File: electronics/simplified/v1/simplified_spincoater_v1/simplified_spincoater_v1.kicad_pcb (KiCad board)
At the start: 6 copper layers, 49.7 x 49.6 mm, 91 parts, among them U1 HUSB238A-BB001-QN16R, U10 TJA1051TK/3, U11 NTTFS5C454NL, U13 NTTFS5C454NL, U14 NTTFS5C454NL, U15 NTTFS5C454NL, U16 NTTFS5C454NL, U17 NTTFS5C454NL, U18 TJA1051TK/3, U2 LMR51420YDD, U3 TPS62933DRL, U4 GT-USB-7004N, U6 ESP32-S3-WROOM-1, U7 STM32G474VEH6, U8 DRV8323SRTA, U9 AS5600

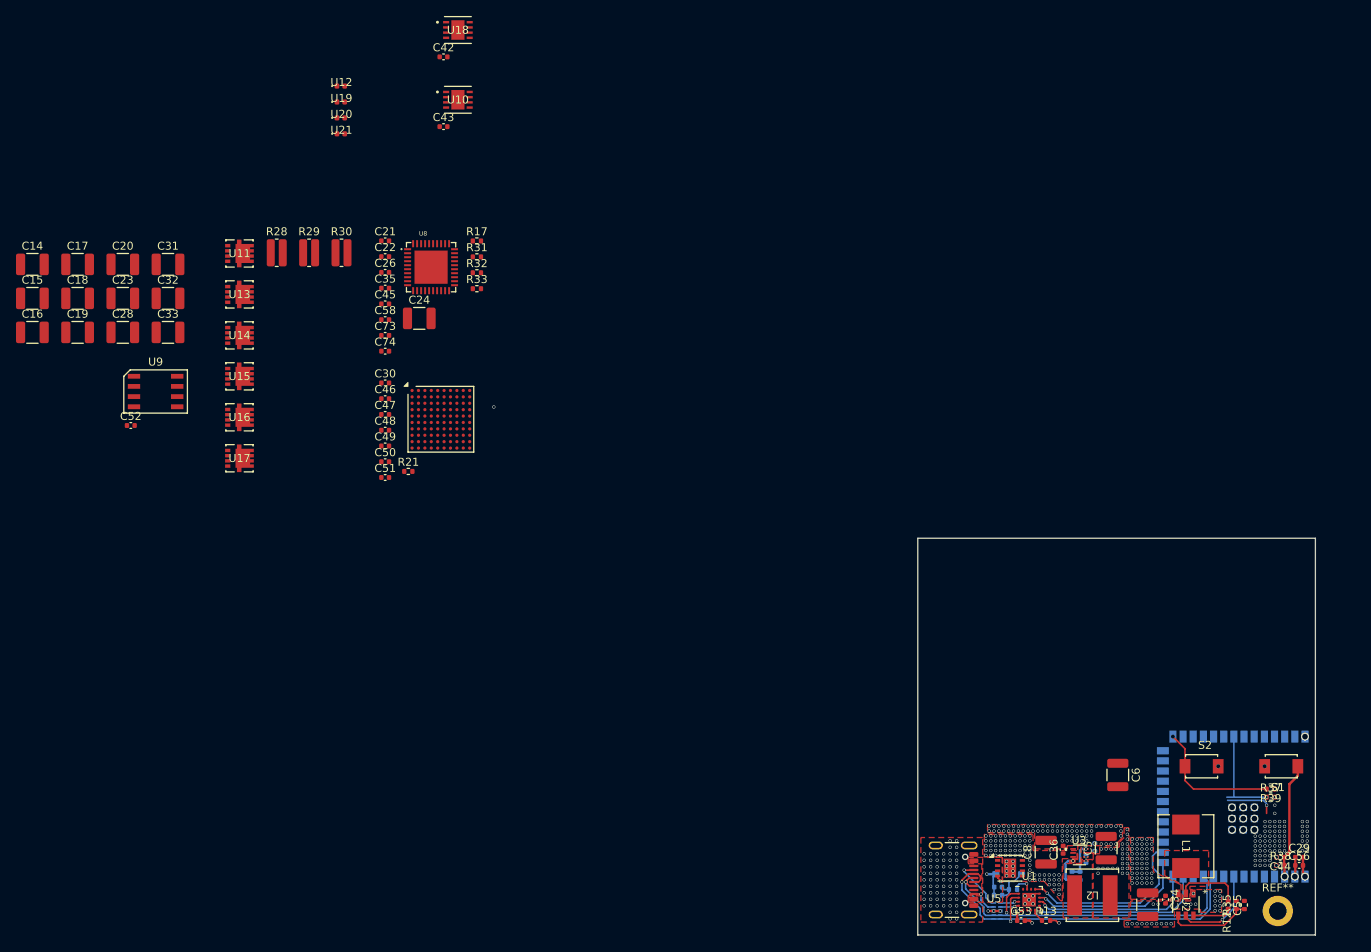
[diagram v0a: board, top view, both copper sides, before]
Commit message: fix
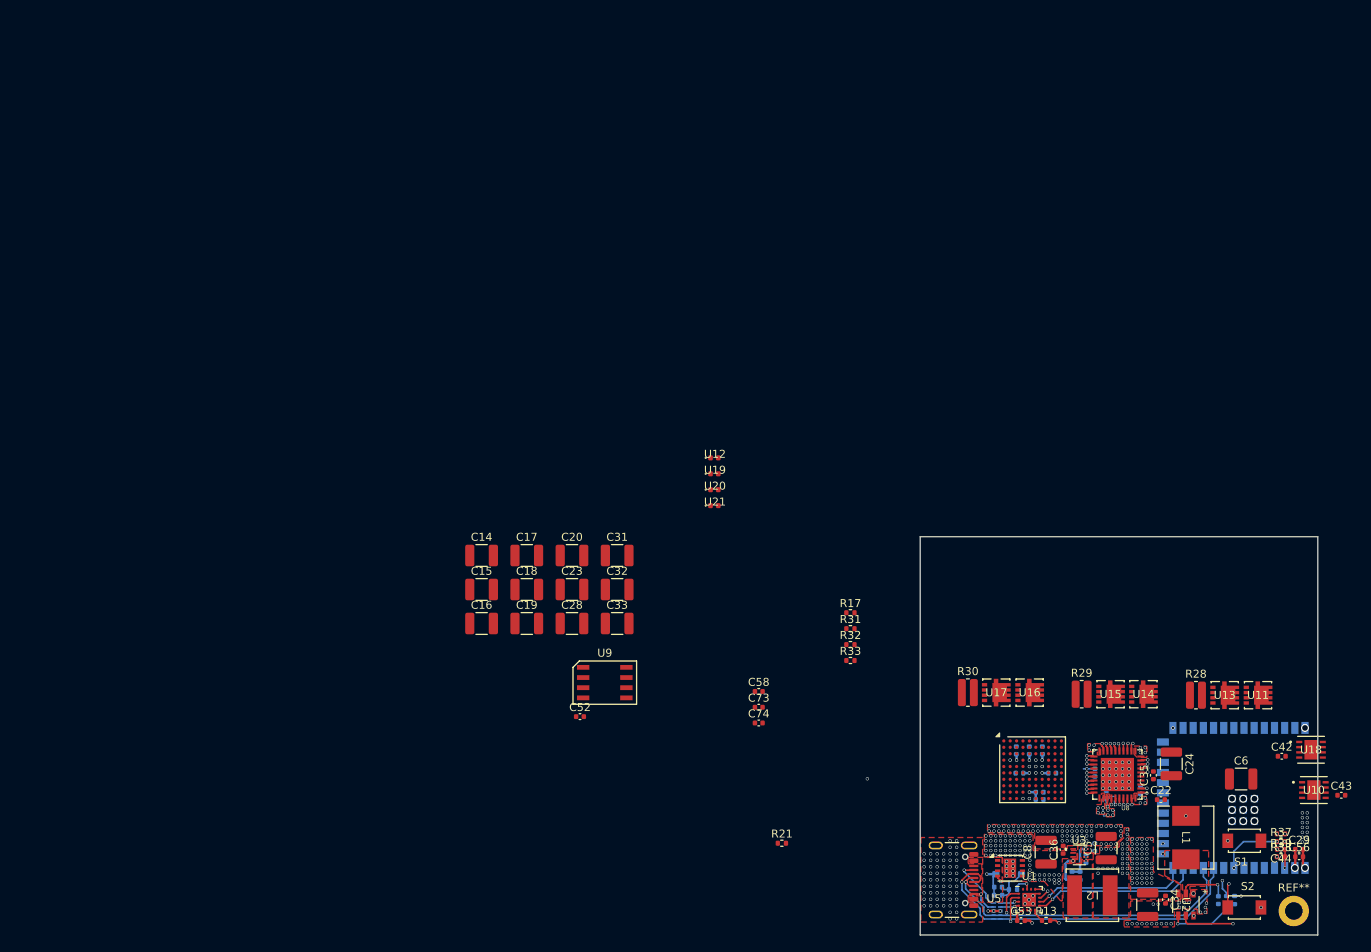
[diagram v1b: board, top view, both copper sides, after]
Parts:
- C21, C26, C30, C45, C46, C47, C48, C49, C50, C51, C55, R12, R35: moved to B.Cu
- moved C43 139.9 mm to (165.9, 97.5)
- moved U18 139.5 mm to (162.2, 91.8)
- moved U11 138.8 mm to (155.5, 85.0)
- moved U10 137.5 mm to (162.5, 96.9)
- moved C42 136.5 mm to (158.5, 92.7)
- moved U13 133.0 mm to (151.4, 85.0)
- moved R28 127.5 mm to (147.8, 85.0)
- moved U14 121.6 mm to (141.2, 84.9)
- moved C22 118.4 mm to (143.4, 98.1)
- moved C21 116.7 mm to (140.8, 96.9), turned to -90 degrees
- moved U15 115.9 mm to (137.1, 84.9)
- moved C35 113.7 mm to (142.5, 95.0), turned to 90 degrees
- moved C26 111.3 mm to (136.6, 97.5), turned to 90 degrees
- moved R29 111.2 mm to (133.5, 84.9)
- moved C24 109.3 mm to (144.7, 93.6), turned to -90 degrees
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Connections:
- net /motor/Gate Driver/GATE_DRIVER_NFALUT renamed /motor/Gate Driver/GATE_DRIVER_NFAULT
- U6 pad 41_1: (no net) -> GND
- U6 pad 41_2: (no net) -> GND
- U6 pad 41_3: (no net) -> GND
- U6 pad 41_4: (no net) -> GND
- U6 pad 41_5: (no net) -> GND
- U6 pad 41_6: (no net) -> GND
- U6 pad 41_7: (no net) -> GND
- U6 pad 41_8: (no net) -> GND
- U6 pad 41_9: (no net) -> GND
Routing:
- net Net-(U6-IO0): track 16.8 -> 35.6 mm, vias 1 -> 3
- net +12V: track 0.00 -> 12.1 mm, vias 1 -> 2
- net Net-(U6-EN): track 14.6 -> 2.63 mm
- net +3V3: track 4.84 -> 11.9 mm, vias 32 -> 40
- net Net-(U2-FB): track 16.5 -> 9.53 mm
- net Net-(U2-CB): track 5.08 -> 0.15 mm, vias 0 -> 1
- net /motor/Gate Driver/GATE_DRIVER_INLA: track 0.00 -> 2.52 mm, vias 0 -> 3
- net Net-(U8-DVDD): track 0.00 -> 2.13 mm, vias 0 -> 5
- net Net-(U2-SW): track 8.37 -> 6.39 mm, vias 0 -> 1
- net Net-(U8-CPL): track 0.00 -> 1.74 mm, vias 0 -> 1
- net /MCU/EN_12V: track 23.7 -> 22.0 mm, vias 2 -> 3
- net Net-(U8-CPH): track 0.00 -> 1.69 mm, vias 0 -> 1
- net /MCU/PD_FAULT: track 22.5 -> 21.1 mm, vias 1 -> 2
- net /MCU/PD_SCL: track 20.8 -> 19.4 mm
- net /MCU/PD_SDA: track 22.1 -> 20.8 mm
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- added copper zone on In1.Cu, net GND
- added copper zone on In4.Cu, net GND
- added copper zone on B.Cu, net Net-(U8-DVDD)
- added copper zone on F.Cu, net Net-(U8-DVDD)
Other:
- board size 49.7 x 49.6 mm -> 49.7 x 49.8 mm
